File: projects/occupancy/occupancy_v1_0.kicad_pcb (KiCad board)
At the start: 2 copper layers, 53.5 x 59 mm, 18 parts, among them J1 Conn_01x01, J2 Conn_01x03_Female, J3 Conn_01x01, J4 Conn_01x01, J5 Conn_01x01, K1 JQC-3F-1C-DC5V, Q1 BC547, U1 Easy-Power, U2 LM555

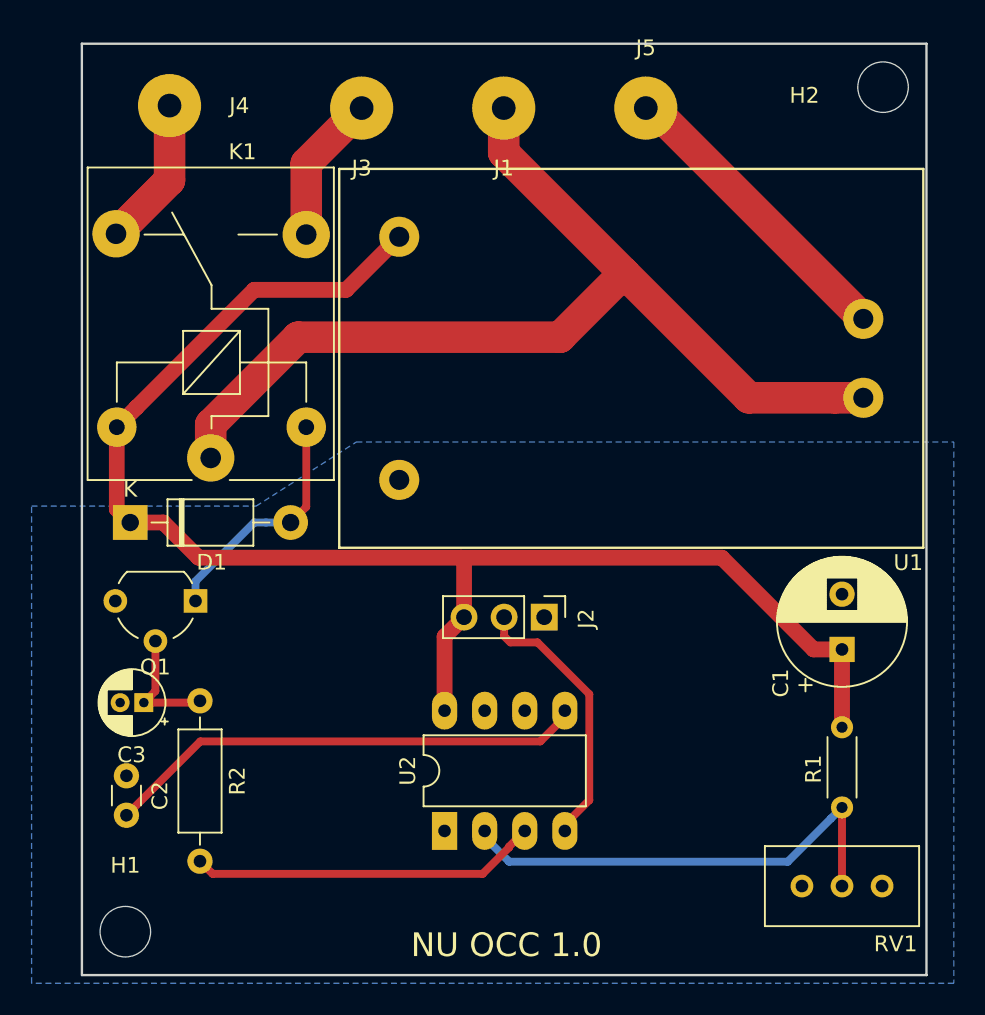
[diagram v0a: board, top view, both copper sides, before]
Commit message: Cost XLS and v1.1 and changes
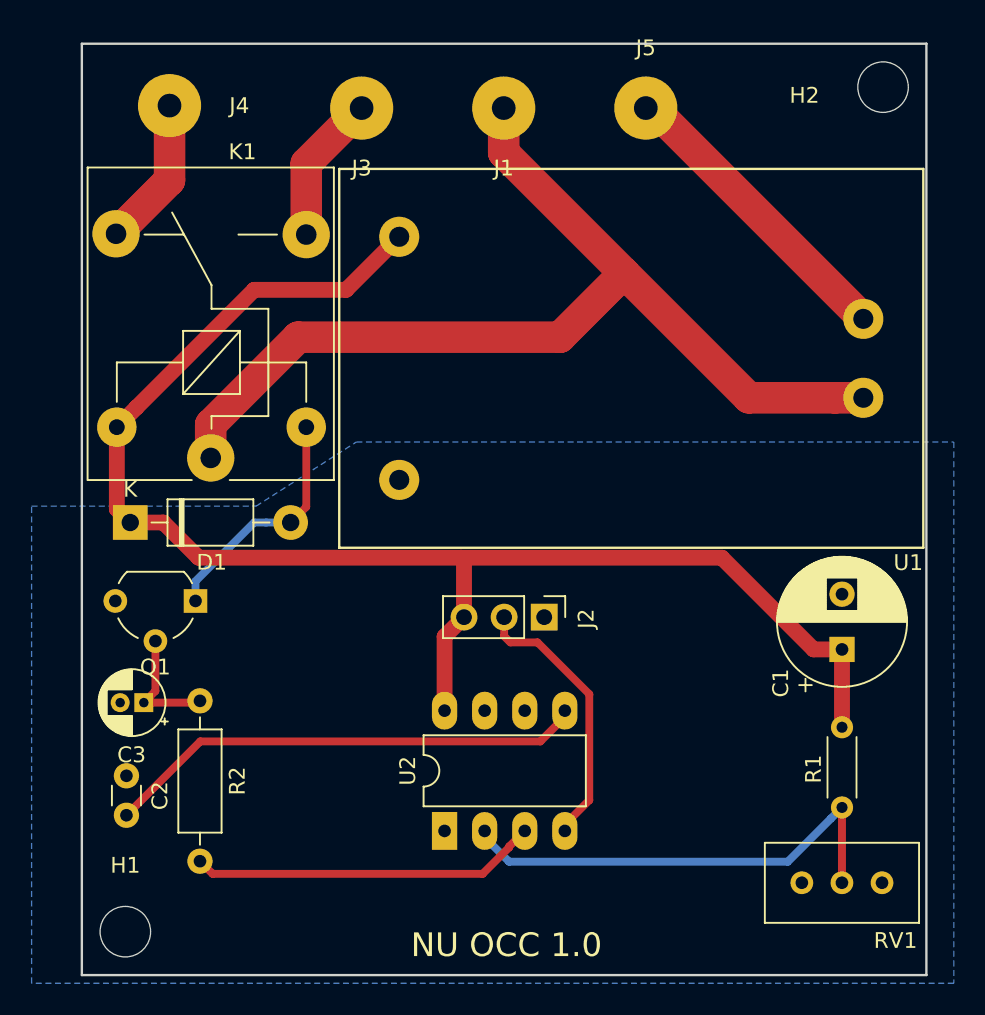
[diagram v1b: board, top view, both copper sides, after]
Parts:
- C1: value 470uF -> 470uF,16V
- C3: value 10uF -> 10uF,16V
- U2: value LM555 -> NE555
- moved RV1 0.21 mm to (158.0, 140.9)
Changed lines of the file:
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@@
   (general
     (thickness 1.6)
-    (drawings 32)
-    (tracks 66)
+    (drawings 34)
+    (tracks 67)
     (zones 0)
     (modules 18)
@@
       (effects (font (size 1 1) (thickness 0.15)))
     )
-    (fp_text value 470uF (at -3.81 0 180) (layer F.Fab)
+    (fp_text value 470uF,16V (at -3.81 0 180) (layer F.Fab)
       (effects (font (size 1 1) (thickness 0.15)))
     )
@@
       (effects (font (size 1 1) (thickness 0.15)))
     )
-    (fp_text value 10uF (at 5.08 1.27 180) (layer F.Fab)
+    (fp_text value 10uF,16V (at 5.08 1.27 180) (layer F.Fab)
       (effects (font (size 1 1) (thickness 0.15)))
     )
@@
   )
   (module Potentiometer_THT:Potentiometer_Bourns_3296W_Vertical (layer F.Cu)
-    (at 158.02 141.16)
+    (at 158.015 140.95)
     (descr "Potentiometer, vertical, Bourns 3296W, https://www.bourns.com/pdfs/3296.pdf")
     (tags "Potentiometer vertical Bourns 3296W")
@@
       (effects (font (size 1 1) (thickness 0.15)))
     )
-    (fp_text value LM555 (at 3.81 9.95 90) (layer F.Fab)
+    (fp_text value NE555 (at 3.81 9.95 90) (layer F.Fab)
       (effects (font (size 1 1) (thickness 0.15)))
     )
@@
       (net 12 "Net-(J5-Pad1)"))
   )
-  (dimension 8.900035 (width 0.3) (layer Dwgs.User)
-    (gr_text "8.900 mm" (at 156.320725 177.134406 359.8390572) (layer Dwgs.User)
+  (gr_arc (start 160.825 146.8) (end 160.825 143.8) (angle -90) (layer Dwgs.User) (width 0.15))
+  (gr_arc (start 107.325 87.8) (end 107.325 90.8) (angle -90) (layer Dwgs.User) (width 0.15))
+  (dimension 8.900035 (width 0.3) (layer Cmts.User)
+    (gr_text "8.900 mm" (at 156.320725 177.134406 359.8390572) (layer Cmts.User)
       (effects (font (size 1.5 1.5) (thickness 0.3)))
     )
@@
     (arrow2b (pts (xy 151.876624 175.021914) (xy 153.004771 174.43866)))
   )
-  (dimension 6.800184 (width 0.3) (layer Dwgs.User)
-    (gr_text "6.800 mm" (at 193.969108 143.708964 89.5787151) (layer Dwgs.User)
+  (dimension 6.875 (width 0.3) (layer Cmts.User)
+    (gr_text "6.875 mm" (at 193.95108 143.4375 270) (layer Cmts.User)
       (effects (font (size 1.5 1.5) (thickness 0.3)))
     )
-    (feature1 (pts (xy 151.925 146.8) (xy 192.43057 147.097835)))
-    (feature2 (pts (xy 151.975 140) (xy 192.48057 140.297835)))
-    (crossbar (pts (xy 191.894165 140.293523) (xy 191.844165 147.093523)))
-    (arrow1a (pts (xy 191.844165 147.093523) (xy 191.266043 145.962738)))
-    (arrow1b (pts (xy 191.844165 147.093523) (xy 192.438853 145.971361)))
-    (arrow2a (pts (xy 191.894165 140.293523) (xy 191.299477 141.415685)))
-    (arrow2b (pts (xy 191.894165 140.293523) (xy 192.472287 141.424308)))
-  )
-  (dimension 5.300059 (width 0.3) (layer Dwgs.User)
-    (gr_text "5.300 mm" (at 158.28125 161.462494 0.2702611065) (layer Dwgs.User)
+    (feature1 (pts (xy 151.975 146.875) (xy 192.437501 146.875)))
+    (feature2 (pts (xy 151.975 140) (xy 192.437501 140)))
+    (crossbar (pts (xy 191.85108 140) (xy 191.85108 146.875)))
+    (arrow1a (pts (xy 191.85108 146.875) (xy 191.264659 145.748496)))
+    (arrow1b (pts (xy 191.85108 146.875) (xy 192.437501 145.748496)))
+    (arrow2a (pts (xy 191.85108 140) (xy 191.264659 141.126504)))
+    (arrow2b (pts (xy 191.85108 140) (xy 192.437501 141.126504)))
+  )
+  (dimension 5.300059 (width 0.3) (layer Cmts.User)
+    (gr_text "5.300 mm" (at 158.28125 161.462494 0.2702611065) (layer Cmts.User)
       (effects (font (size 1.5 1.5) (thickness 0.3)))
     )
@@
   )
   (gr_line (start 151.05 138.85) (end 152.9 141.15) (layer Dwgs.User) (width 0.15))
-  (dimension 26.700105 (width 0.3) (layer Dwgs.User)
-    (gr_text "26.700 mm" (at 147.474788 155.587017 0.1609427776) (layer Dwgs.User)
+  (dimension 26.700105 (width 0.3) (layer Cmts.User)
+    (gr_text "26.700 mm" (at 147.474788 155.587017 0.1609427776) (layer Cmts.User)
       (effects (font (size 1.5 1.5) (thickness 0.3)))
     )
@@
     (arrow2b (pts (xy 134.118889 153.524525) (xy 135.243741 152.934942)))
   )
-  (dimension 26.775 (width 0.3) (layer Dwgs.User)
-    (gr_text "26.775 mm" (at 120.6875 155.55) (layer Dwgs.User)
+  (dimension 26.700012 (width 0.3) (layer Cmts.User)
+    (gr_text "26.700 mm" (at 120.641784 155.587496 -0.05364771795) (layer Cmts.User)
       (effects (font (size 1.5 1.5) (thickness 0.3)))
     )
-    (feature1 (pts (xy 107.3 146.8) (xy 107.3 154.036421)))
-    (feature2 (pts (xy 134.075 146.8) (xy 134.075 154.036421)))
-    (crossbar (pts (xy 134.075 153.45) (xy 107.3 153.45)))
-    (arrow1a (pts (xy 107.3 153.45) (xy 108.426504 152.863579)))
-    (arrow1b (pts (xy 107.3 153.45) (xy 108.426504 154.036421)))
-    (arrow2a (pts (xy 134.075 153.45) (xy 132.948496 152.863579)))
-    (arrow2b (pts (xy 134.075 153.45) (xy 132.948496 154.036421)))
-  )
-  (dimension 13.175024 (width 0.3) (layer Dwgs.User)
-    (gr_text "13.175 mm" (at 177.237494 140.294379 89.89127949) (layer Dwgs.User)
+    (feature1 (pts (xy 107.3 146.8) (xy 107.293201 154.061418)))
+    (feature2 (pts (xy 134 146.825) (xy 133.993201 154.086418)))
+    (crossbar (pts (xy 133.99375 153.499997) (xy 107.29375 153.474997)))
+    (arrow1a (pts (xy 107.29375 153.474997) (xy 108.420802 152.889631)))
+    (arrow1b (pts (xy 107.29375 153.474997) (xy 108.419704 154.062472)))
+    (arrow2a (pts (xy 133.99375 153.499997) (xy 132.867796 152.912522)))
+    (arrow2b (pts (xy 133.99375 153.499997) (xy 132.866698 154.085363)))
+  )
+  (dimension 13.200095 (width 0.3) (layer Cmts.User)
+    (gr_text "13.200 mm" (at 177.224762 140.388446 89.78297157) (layer Cmts.User)
       (effects (font (size 1.5 1.5) (thickness 0.3)))
     )
-    (feature1 (pts (xy 134.1 133.625) (xy 175.736418 133.704006)))
-    (feature2 (pts (xy 134.075 146.8) (xy 175.711418 146.879006)))
-    (crossbar (pts (xy 175.124998 146.877894) (xy 175.149998 133.702894)))
-    (arrow1a (pts (xy 175.149998 133.702894) (xy 175.73428 134.830508)))
-    (arrow1b (pts (xy 175.149998 133.702894) (xy 174.561441 134.828283)))
-    (arrow2a (pts (xy 175.124998 146.877894) (xy 175.713555 145.752505)))
-    (arrow2b (pts (xy 175.124998 146.877894) (xy 174.540716 145.75028)))
+    (feature1 (pts (xy 134.1 133.625) (xy 175.736193 133.782713)))
+    (feature2 (pts (xy 134.05 146.825) (xy 175.686193 146.982713)))
+    (crossbar (pts (xy 175.099777 146.980492) (xy 175.149777 133.780492)))
+    (arrow1a (pts (xy 175.149777 133.780492) (xy 175.731927 134.909209)))
+    (arrow1b (pts (xy 175.149777 133.780492) (xy 174.559093 134.904766)))
+    (arrow2a (pts (xy 175.099777 146.980492) (xy 175.690461 145.856218)))
+    (arrow2b (pts (xy 175.099777 146.980492) (xy 174.517627 145.851775)))
   )
   (gr_line (start 122.6 122.1) (end 145.6 122.1) (layer Dwgs.User) (width 0.15))
@@
     (effects (font (size 1.5 1.5) (thickness 0.3)))
   )
-  (gr_line (start 107.325 87.8) (end 160.83 87.8) (layer Edge.Cuts) (width 0.15))
-  (gr_line (start 107.33 146.8) (end 107.325 87.8) (layer Edge.Cuts) (width 0.15))
-  (gr_line (start 160.83 146.8) (end 107.33 146.8) (layer Edge.Cuts) (width 0.15))
-  (gr_line (start 160.83 87.8) (end 160.83 146.8) (layer Edge.Cuts) (width 0.15))
+  (gr_line (start 107.325 87.8) (end 160.825 87.8) (layer Edge.Cuts) (width 0.15))
+  (gr_line (start 107.325 146.8) (end 107.325 87.8) (layer Edge.Cuts) (width 0.15))
+  (gr_line (start 160.825 146.8) (end 107.325 146.8) (layer Edge.Cuts) (width 0.15))
+  (gr_line (start 160.825 87.8) (end 160.825 146.8) (layer Edge.Cuts) (width 0.15))
   (segment (start 110.789999 110.840001) (end 109.54 112.09) (width 1) (layer F.Cu) (net 1))
   (segment (start 124.069999 103.390001) (end 118.239999 103.390001) (width 1) (layer F.Cu) (net 1))
@@
   (segment (start 137.922 137.268) (end 139.47201 135.71799) (width 0.5) (layer F.Cu) (net 7))
   (segment (start 137.922 137.668) (end 137.922 137.268) (width 0.5) (layer F.Cu) (net 7))
-  (segment (start 155.48 136.18) (end 155.48 141.16) (width 0.5) (layer F.Cu) (net 8))
   (segment (start 154.780001 136.879999) (end 155.48 136.18) (width 0.5) (layer B.Cu) (net 8))
   (segment (start 152.04199 139.61801) (end 154.780001 136.879999) (width 0.5) (layer B.Cu) (net 8))
@@
   (segment (start 132.842 138.068) (end 134.39201 139.61801) (width 0.5) (layer B.Cu) (net 8))
   (segment (start 132.842 137.668) (end 132.842 138.068) (width 0.5) (layer B.Cu) (net 8))
+  (segment (start 155.475 136.185) (end 155.48 136.18) (width 0.5) (layer F.Cu) (net 8))
+  (segment (start 155.475 140.95) (end 155.475 136.185) (width 0.5) (layer F.Cu) (net 8))
   (segment (start 135.382 137.668) (end 135.382 138.068) (width 0.5) (layer F.Cu) (net 9))
   (segment (start 115.607999 140.385999) (end 114.808 139.586) (width 0.5) (layer F.Cu) (net 9))
